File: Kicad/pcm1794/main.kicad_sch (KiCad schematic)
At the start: 45 parts, among them K1 IOUTL, K2 I2S, K3 MCU, K4 IOUTR, K5 CLOCK, K6 VCC, U1 PCM1794, U2 BD933N1WG, U3 BD950N1G, U4 BD950N1G

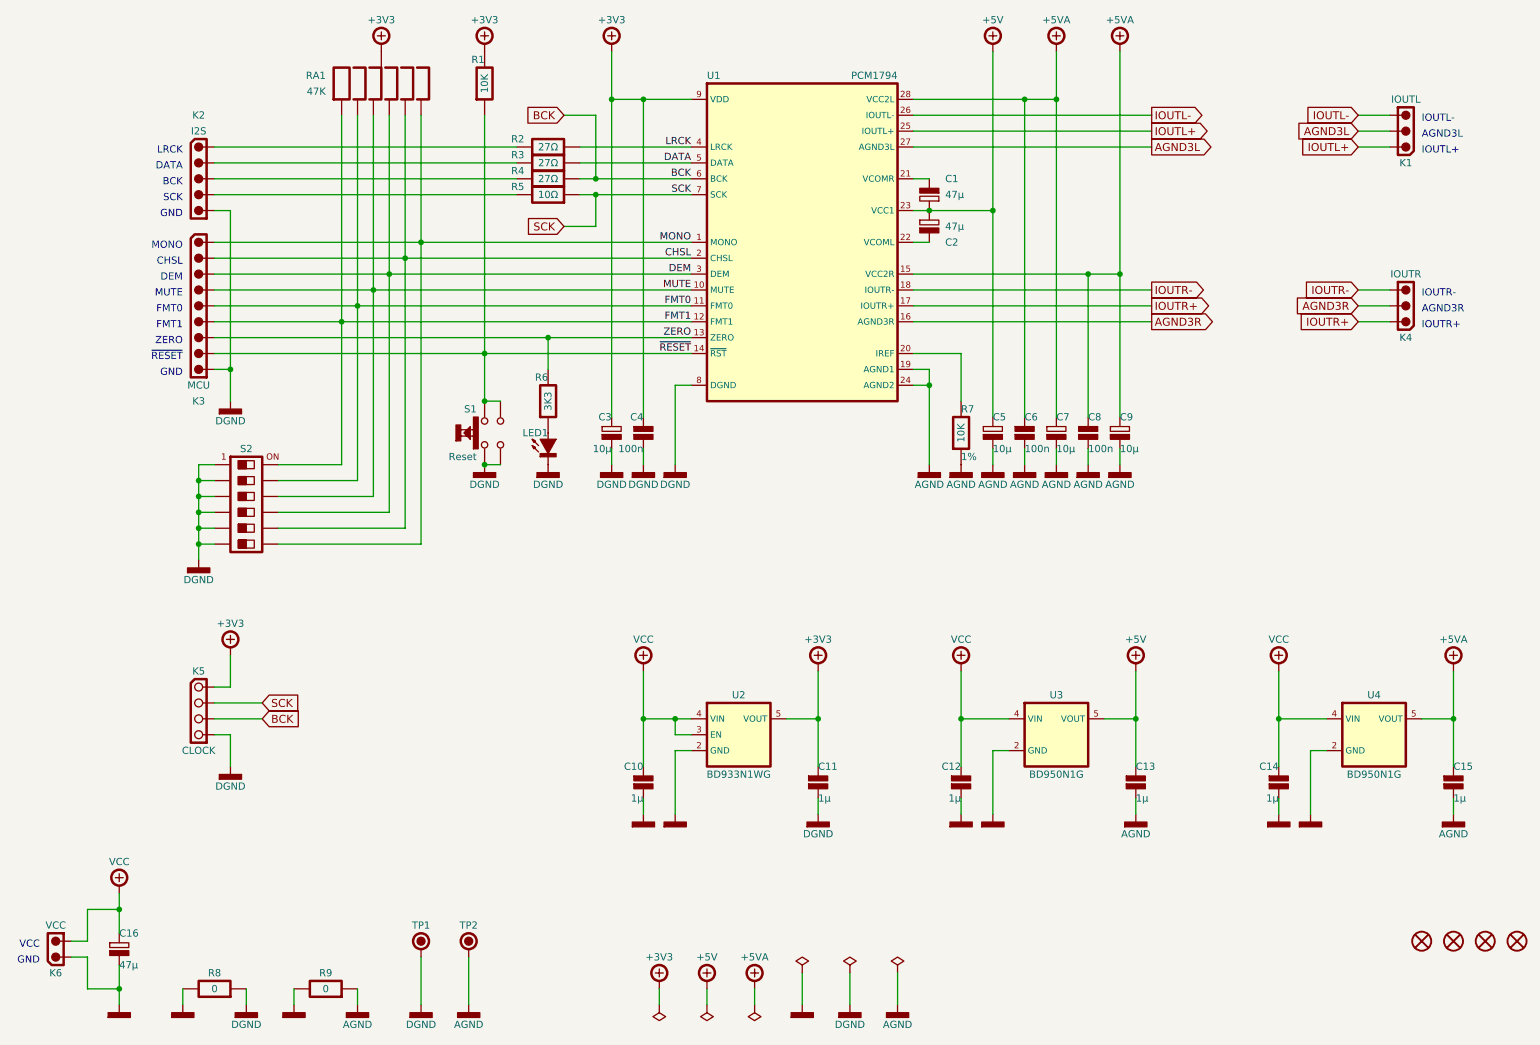
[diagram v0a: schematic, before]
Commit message: Up
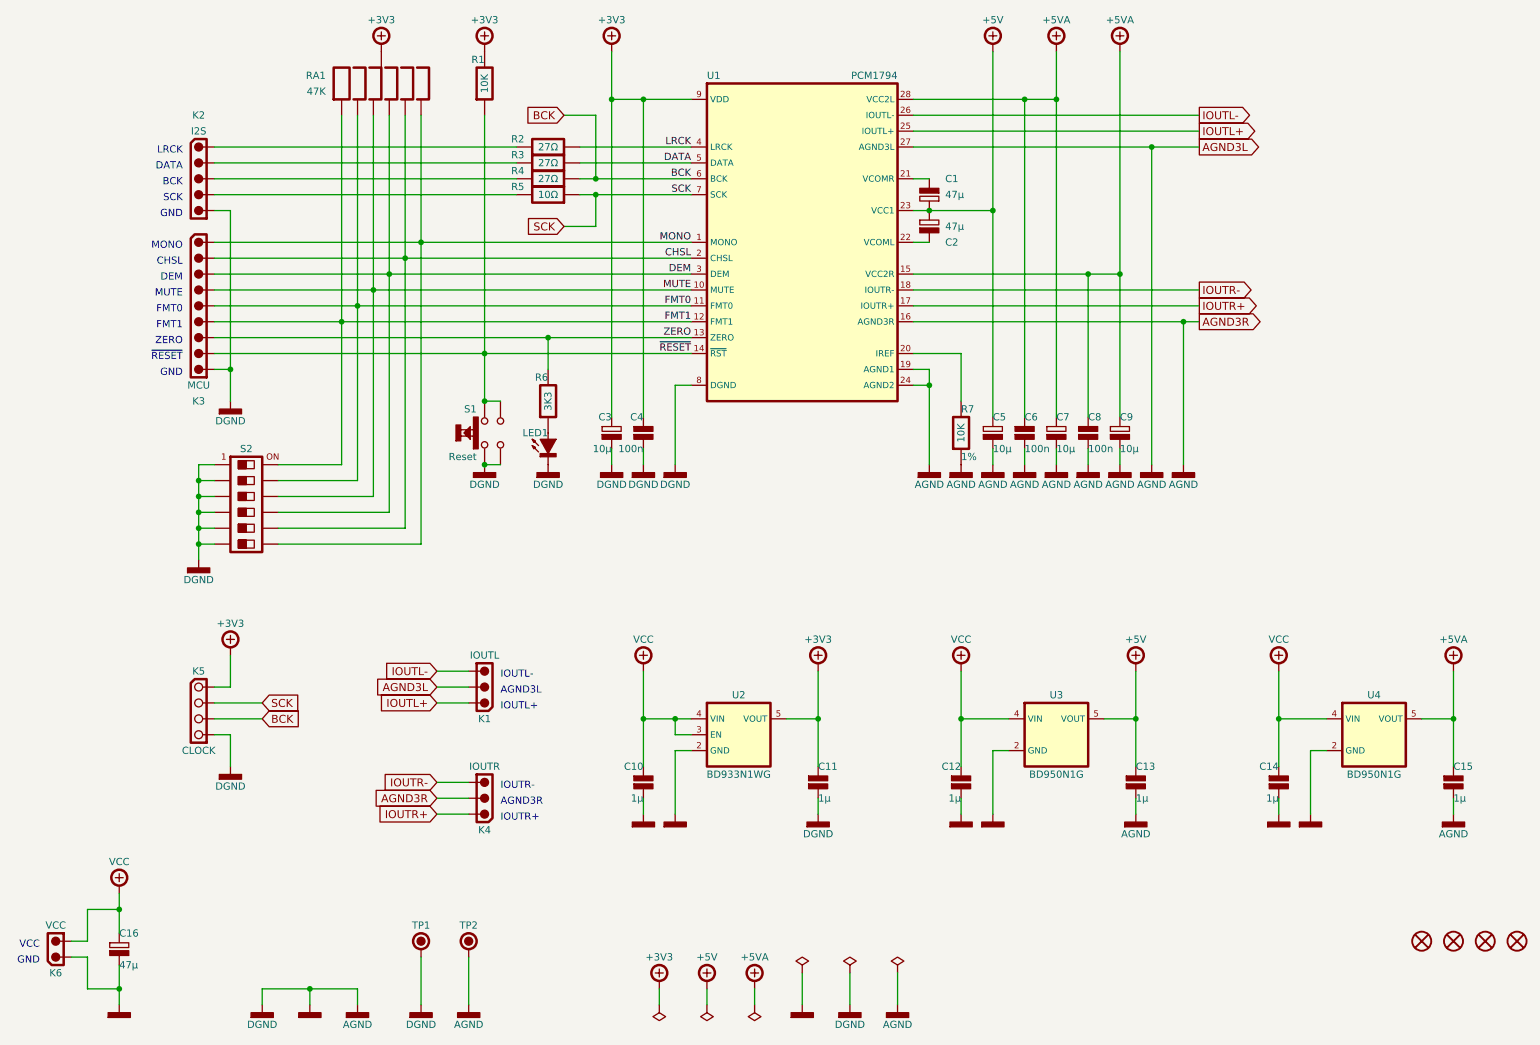
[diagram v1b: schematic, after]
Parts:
- removed R8, R9: 0, tronixio:RESISTOR-SMD-1206, symbol tronixio:KOASPEER-RK73B-1206-0
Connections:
- net AGND3L is gone; now on net AGND: K1.2, U1.27 (AGND3L)
- net AGND3R is gone; now on net AGND: K4.2, U1.16 (AGND3R)
- net DGND is gone; now on net AGND: C11.2, C3.2, C4.2, K2.5, K3.9, K5.4, LED1.1 (C), S1.1, S1.2, S2.1, S2.2, S2.3, S2.4, S2.5, S2.6, TP1.1, U1.8 (DGND)
- net GND is gone; now on net AGND: C10.2, C12.2, C14.2, C16.2, K6.1, U2.2 (GND), U3.2 (GND), U4.2 (GND)
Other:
- moved on the sheet: K1, K4
